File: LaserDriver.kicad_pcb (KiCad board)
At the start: 2 copper layers, 40.2 x 40.5 mm, 31 parts, among them J100 Screw_Terminal_01x04, J101 Screw_Terminal_01x02, J102 nano_left, J103 nano_right, U100 TPS92513DGQR

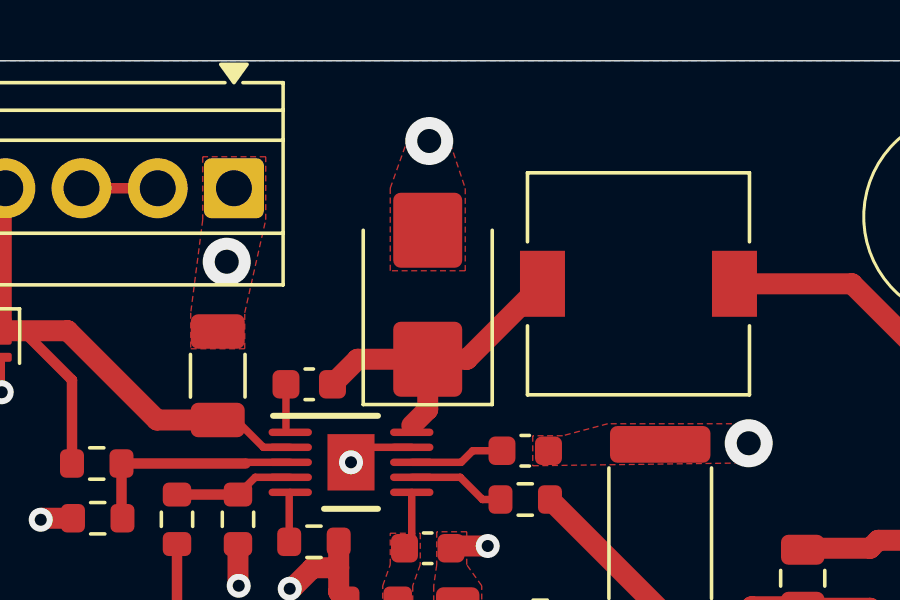
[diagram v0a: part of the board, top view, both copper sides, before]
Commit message: created gerber and assembly files
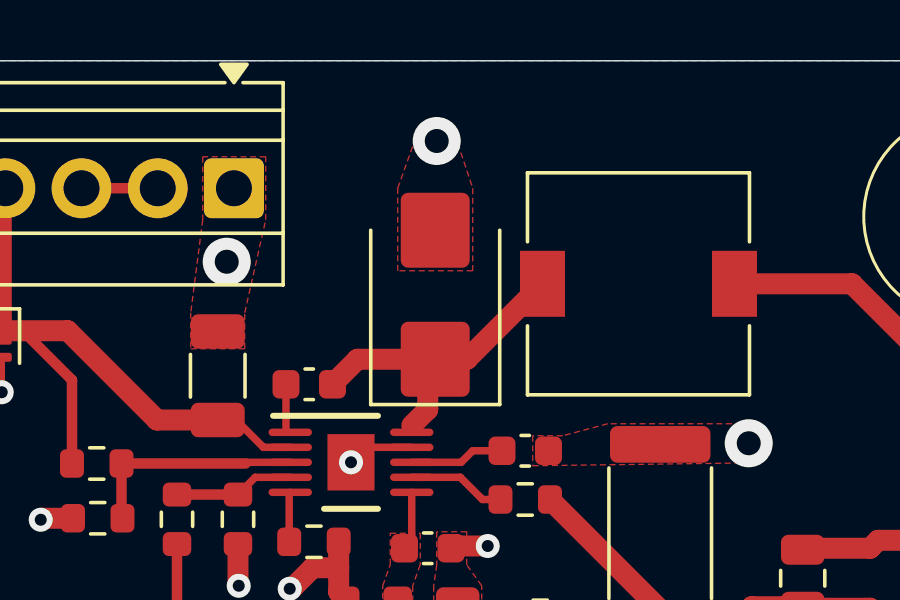
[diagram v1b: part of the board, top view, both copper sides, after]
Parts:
- moved D101 0.25 mm to (46.2, 104.8)
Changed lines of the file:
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@@
 			(usegerberattributes yes)
 			(usegerberadvancedattributes yes)
-			(creategerberjobfile yes)
+			(creategerberjobfile no)
 			(dashed_line_dash_ratio 12.000000)
 			(dashed_line_gap_ratio 3.000000)
@@
 			(outputformat 1)
 			(mirror no)
-			(drillshape 1)
+			(drillshape 0)
 			(scaleselection 1)
-			(outputdirectory "")
+			(outputdirectory "Gerbers/")
 		)
 	)
@@
 	(footprint "Diode_SMD:D_SMB"
 		(layer "F.Cu")
-		(at 46 104.8 90)
+		(at 46.25 104.8 90)
 		(descr "Diode SMB (DO-214AA)")
 		(tags "Diode SMB (DO-214AA)")
@@
 	)
 	(via
-		(at 46.05 99.675)
+		(at 46.3 99.675)
 		(size 1.6)
 		(drill 0.8)
@@
 	)
 	(segment
-		(start 47.31 106.95)
-		(end 49.825 104.435)
+		(start 43.66 106.95)
+		(end 42.825 107.785)
 		(width 0.7)
 		(layer "F.Cu")
@@
 	)
 	(segment
-		(start 46 106.95)
-		(end 43.66 106.95)
+		(start 46.25 106.95)
+		(end 46 107.2)
 		(width 0.7)
 		(layer "F.Cu")
@@
 	)
 	(segment
-		(start 43.66 106.95)
-		(end 42.825 107.785)
+		(start 46 108.626498)
+		(end 45.467501 109.158997)
 		(width 0.7)
 		(layer "F.Cu")
@@
 	)
 	(segment
-		(start 46 106.95)
-		(end 47.31 106.95)
+		(start 47.31 106.95)
+		(end 46.25 106.95)
 		(width 0.7)
 		(layer "F.Cu")
@@
 	)
 	(segment
-		(start 46 106.95)
+		(start 46 107.2)
 		(end 46 108.626498)
 		(width 0.7)
@@
 	)
 	(segment
-		(start 46 108.626498)
-		(end 45.467501 109.158997)
+		(start 49.825 104.435)
+		(end 47.31 106.95)
+		(width 0.7)
+		(layer "F.Cu")
+		(net 4)
+	)
+	(segment
+		(start 46.25 106.95)
+		(end 43.66 106.95)
 		(width 0.7)
 		(layer "F.Cu")
@@
 		(polygon
 			(pts
-				(xy 47.25 104) (xy 44.75 104) (xy 44.75 101.25) (xy 45.5 99.15) (xy 46.55 99.15) (xy 47.25 101.25)
+				(xy 47.5 104) (xy 45 104) (xy 45 101.25) (xy 45.75 99.15) (xy 46.8 99.15) (xy 47.5 101.25)
 			)
 		)
